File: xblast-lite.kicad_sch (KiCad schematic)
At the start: 15 parts, among them J1 TC2050, J2 XBOX LPC, J3 GPIO, J4 LCD, J5 PLCC-32 Socket, U1 74LVC125, U2 SST49LF080A-33-4C-NHE, U3 XC9572XL-xxVQx44, U4 TPS27081A

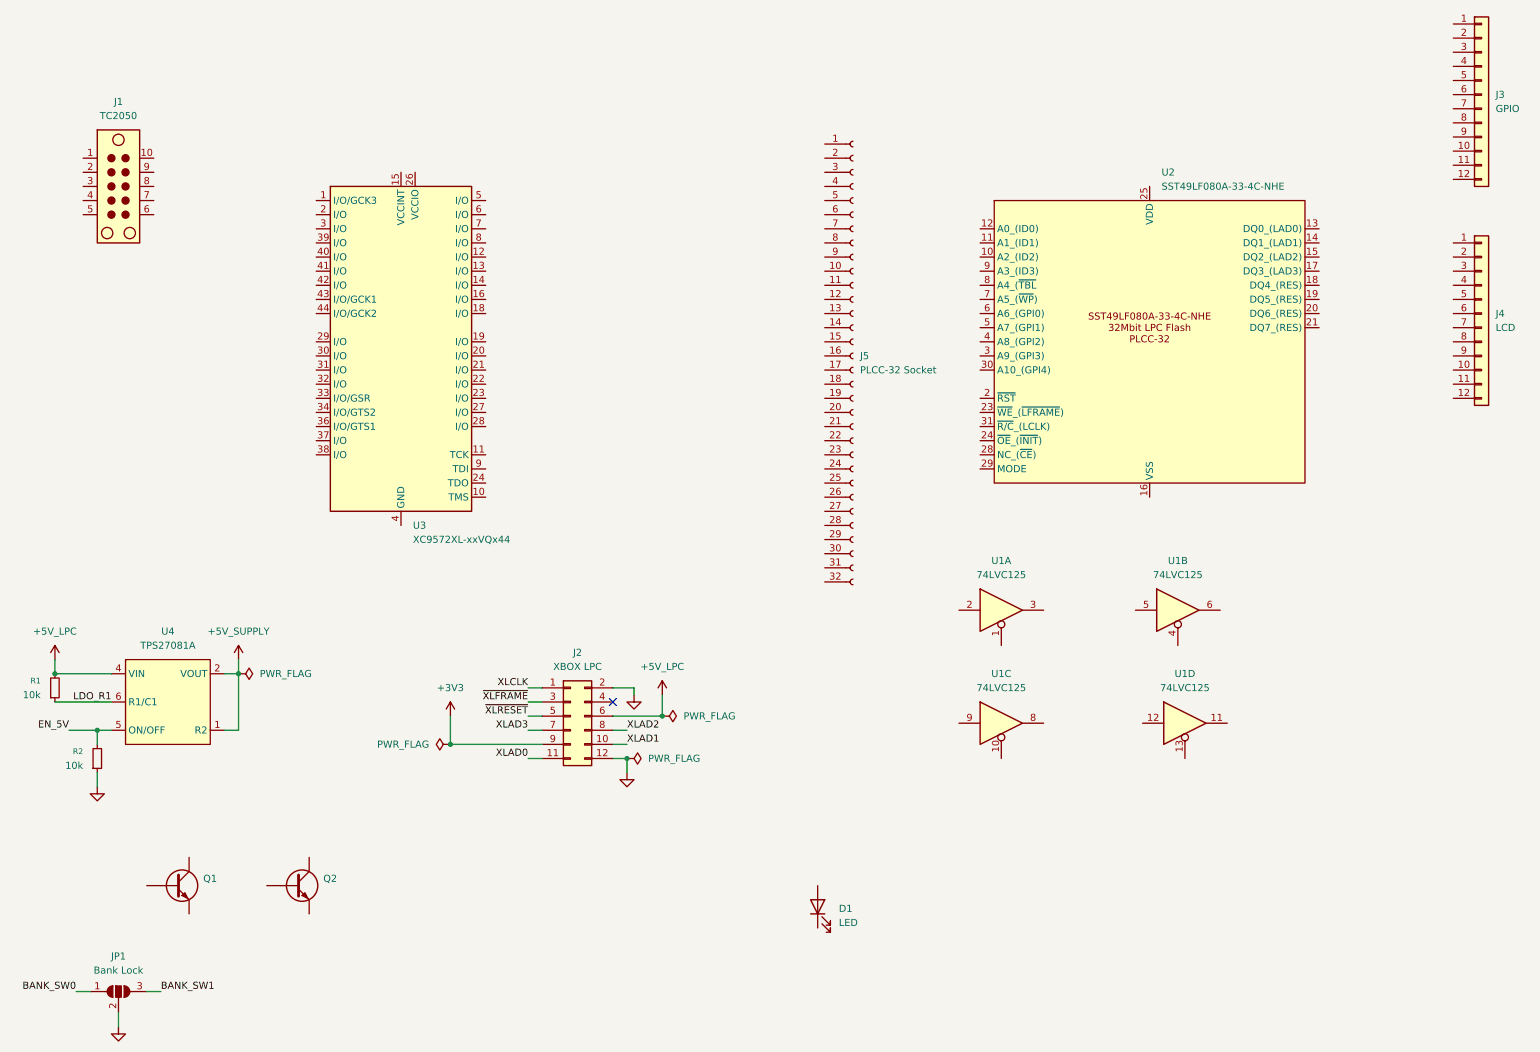
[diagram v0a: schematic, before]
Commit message: More work, initial layout
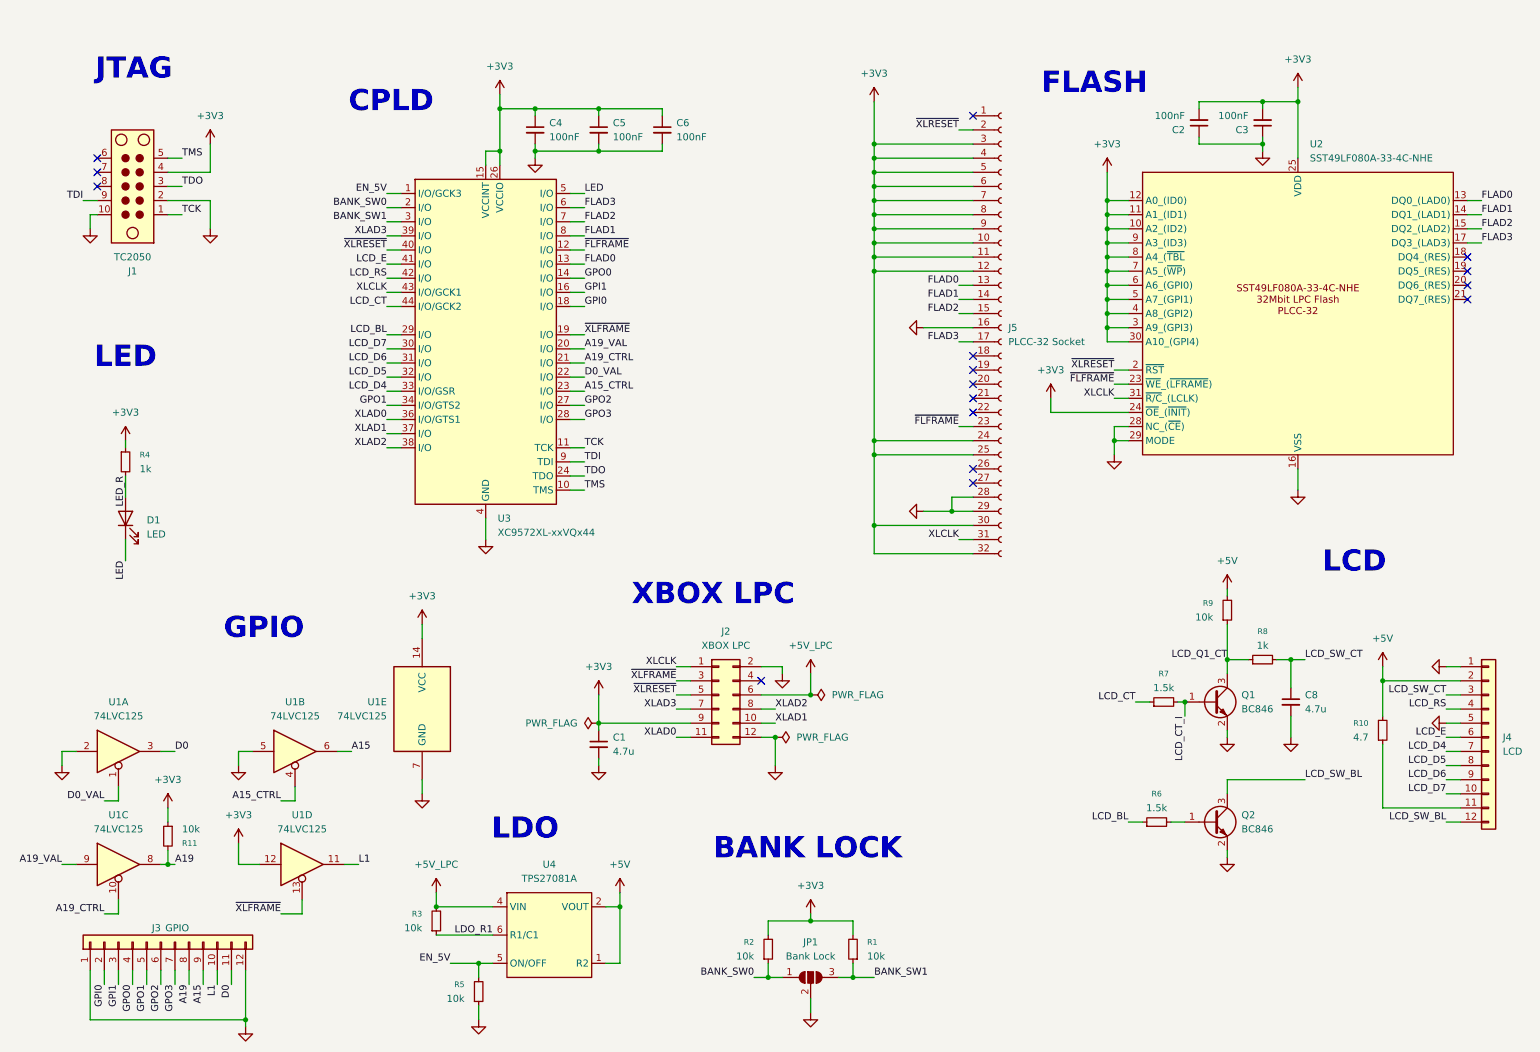
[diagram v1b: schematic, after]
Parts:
- added C1, C8: 4.7u, Capacitor_SMD:C_0805_2012Metric, symbol Device:C_Small
- added C2, C3, C4, C5, C6: 100nF, Capacitor_SMD:C_0603_1608Metric, symbol Device:C_Small
- added R1, R11, R2, R9: 10k, Resistor_SMD:R_0603_1608Metric, symbol Device:R_Small
- added R10: 4.7, Resistor_SMD:R_0805_2012Metric, symbol Device:R_Small
- added R4, R8: 1k, Resistor_SMD:R_0603_1608Metric, symbol Device:R_Small
- added R6, R7: 1.5k, Resistor_SMD:R_0603_1608Metric, symbol Device:R_Small
- added unit 5 of U1
- D1: footprint (none) -> LED_SMD:LED_0603_1608Metric; Distributor Link 1 (none) -> https://www.digikey.com/en/products/detail/liteon/LTST-C194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; Distributor Link 2 (none) -> https://www.mouser.com/en/ProductDetail/LITEON/LTST-C194KGK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; LCSC (none) -> C913102; Manufacturer (none) -> Lite-On; Manufacturer Part Number (none) -> LTST-C194KGKT
- J2: footprint Connector_PinSocket_2.54mm:PinSocket_2x06_P2.54mm_Vertical -> Connector_PinSocket_2.54mm:PinSocket_2x06_P2.54mm_Vertical_SMD; Distributor Link 1 https://www.digikey.com/en/products/detail/te-connectivity-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 -> https://www.digikey.com/en/products/detail/samtec-inc/SSM-1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; Distributor Link 2 https://www.mouser.com/en/ProductDetail/TE-Connectivity/5-5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 -> https://www.mouser.com/ProductDetail/Samtec/SSM-106-L-DV-BE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; LCSC C18078145 -> C3975151; Manufacturer Bossie -> HCTL; Manufacturer Part Number BX-PM2.54-2-6PY -> PM254-2-06-S-8.5
- J3: footprint Connector_PinSocket_2.54mm:PinSocket_1x12_P2.54mm_Vertical -> xblast-lite:SolderWirePad_1x12_SMD_2x4mm; now left out of the parts list
- Q1, Q2: value (none) -> BC846; symbol Device:Q_NPN -> Transistor_BJT:BC846
- renumbered R1 to R3, R2 to R5
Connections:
- net +5V_SUPPLY is gone; now on net +5V: U4.1 (R2), U4.2 (VOUT), U4.3 (VOUT)
- net +3V3: now also J1.4, J5.10 (Pin_10), J5.11 (Pin_11), J5.12 (Pin_12), J5.24 (Pin_24), J5.25 (Pin_25), J5.3 (Pin_3), J5.30 (Pin_30), J5.32 (Pin_32), J5.4 (Pin_4), J5.5 (Pin_5), J5.6 (Pin_6), J5.7 (Pin_7), J5.8 (Pin_8), J5.9 (Pin_9), U1.12, U2.10 (A2_(ID2)), U2.11 (A1_(ID1)), U2.12 (A0_(ID0)), U2.24 (~{OE}_(~{INIT})), U2.25 (VDD), U2.3 (A9_(GPI3)), U2.30 (A10_(GPI4)), U2.32 (VDD), U2.4 (A8_(GPI2)), U2.5 (A7_(GPI1)), U2.6 (A6_(GPI0)), U2.7 (A5_(~{WP})), U2.8 (A4_(~{TBL}), U2.9 (A3_(ID3)), U3.15 (VCCINT), U3.26 (VCCIO), U3.35 (VCCINT), C1.1, C2.2, C3.2, C4.1, C5.1, C6.1, R1.2, R11.1, R2.2, R4.1, U1.14 (VCC)
- net BANK_SW0: now also U3.2 (I/O), R2.1
- net BANK_SW1: now also U3.3 (I/O), R1.1
- net EN_5V: now also U3.1 (I/O/GCK3)
- net GND: now also J1.10, J1.2, J3.1 (Pin_1), J3.12 (Pin_12), J4.1 (Pin_1), J4.5 (Pin_5), J5.16 (Pin_16), J5.28 (Pin_28), J5.29 (Pin_29), Q1.2 (E), Q2.2 (E), U1.2, U1.5, U2.16 (VSS), U2.28 (NC_(~{CE})), U2.29 (MODE), U3.17 (GND), U3.25 (GND), U3.4 (GND), C1.2, C2.1, C3.1, C4.2, C5.2, C6.2, C8.2, U1.7 (GND)
- net XLAD0: now also U3.36 (I/O/GTS1)
- net XLAD1: now also U3.37 (I/O)
- net XLAD2: now also U3.38 (I/O)
- net XLAD3: now also U3.39 (I/O)
- net XLCLK: now also J5.31 (Pin_31), U2.31 (~{R/C}_(LCLK)), U3.43 (I/O/GCK1)
- net ~{XLFRAME}: now also U1.13, U3.19 (I/O)
- net ~{XLRESET}: now also J5.2 (Pin_2), U2.2 (~{RST}), U3.40 (I/O)
- net LED: now reaches D1.1 (K)
- net LED: now also U3.5 (I/O)
- net LED_R: now reaches D1.2 (A)
- net LED_R: now also R4.2
- net FLAD0: now reaches J5.13 (Pin_13)
- net FLAD0: now also U2.13 (DQ0_(LAD0)), U3.13 (I/O)
- net FLAD1: now reaches J5.14 (Pin_14)
- net FLAD1: now also U2.14 (DQ1_(LAD1)), U3.8 (I/O)
- net FLAD2: now reaches J5.15 (Pin_15)
- net FLAD2: now also U2.15 (DQ2_(LAD2)), U3.7 (I/O)
- net FLAD3: now reaches J5.17 (Pin_17)
- net FLAD3: now also U2.17 (DQ3_(LAD3)), U3.6 (I/O)
- net ~{FLFRAME}: now reaches J5.23 (Pin_23)
- net ~{FLFRAME}: now also U2.23 (~{WE}_(~{LFRAME})), U3.12 (I/O)
- net A15_CTRL: now reaches U1.4
- net A15_CTRL: now also U3.23 (I/O)
- net A15: now reaches U1.6
- net A15: now also J3.9 (Pin_9)
- net L1: now reaches J3.10 (Pin_10)
- net L1: now also U1.11
- net D0: now reaches J3.11 (Pin_11)
- net D0: now also U1.3
- net GPI0: now reaches J3.2 (Pin_2)
- net GPI0: now also U3.18 (I/O)
- net GPI1: now reaches J3.3 (Pin_3)
- net GPI1: now also U3.16 (I/O)
- net GPO0: now reaches J3.4 (Pin_4)
- net GPO0: now also U3.14 (I/O)
- net GPO1: now reaches J3.5 (Pin_5)
- net GPO1: now also U3.34 (I/O/GTS2)
- net GPO2: now reaches J3.6 (Pin_6)
- net GPO2: now also U3.27 (I/O)
- net GPO3: now reaches J3.7 (Pin_7)
- net GPO3: now also U3.28 (I/O)
- net A19: now reaches J3.8 (Pin_8)
- net A19: now also U1.8, R11.2
- net A19_CTRL: now reaches U1.10
- net A19_CTRL: now also U3.21 (I/O)
- net A19_VAL: now reaches U1.9
- net A19_VAL: now also U3.20 (I/O)
- net D0_VAL: now reaches U1.1
- net D0_VAL: now also U3.22 (I/O)
- net TMS: now reaches U3.10 (TMS)
- net TMS: now also J1.5
- net TCK: now reaches U3.11 (TCK)
- net TCK: now also J1.1
- net TDO: now reaches U3.24 (TDO)
- net TDO: now also J1.3
- net LCD_BL: now reaches U3.29 (I/O)
- net LCD_BL: now also R6.1
- net LCD_D7: now reaches U3.30 (I/O)
- net LCD_D7: now also J4.10 (Pin_10)
- net LCD_D6: now reaches U3.31 (I/O)
- net LCD_D6: now also J4.9 (Pin_9)
- net LCD_D5: now reaches U3.32 (I/O)
- net LCD_D5: now also J4.8 (Pin_8)
- net LCD_D4: now reaches U3.33 (I/O/GSR)
- net LCD_D4: now also J4.7 (Pin_7)
- net LCD_E: now reaches U3.41 (I/O)
- net LCD_E: now also J4.6 (Pin_6)
- net LCD_RS: now reaches U3.42 (I/O)
- net LCD_RS: now also J4.4 (Pin_4)
- net LCD_CT: now reaches U3.44 (I/O/GCK2)
- net LCD_CT: now also R7.1
- net TDI: now reaches U3.9 (TDI)
- net TDI: now also J1.9
- net at J4.11 (Pin_11): now also R10.1
- net LCD_SW_BL: now reaches J4.12 (Pin_12)
- net LCD_SW_BL: now also Q2.3 (C)
- net +5V: now reaches J4.2 (Pin_2)
- net +5V: now also R10.2, R9.2
- net LCD_SW_CT: now reaches J4.3 (Pin_3)
- net LCD_SW_CT: now also C8.1, R8.2
- new net: Q2.1 (B), R6.2
- new net LCD_CT_I: Q1.1 (B), R7.2
- new net LCD_Q1_CT: Q1.3 (C), R8.1, R9.1
- no-connect marks 1 -> 16
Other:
- note added: "BANK LOCK"
- note added: "CPLD"
- note added: "FLASH"
- note added: "GPIO"
- note added: "JTAG"
- note added: "LCD"
- note added: "LDO"
- note added: "LED"
- note added: "XBOX LPC"
- moved on the sheet: D1, J1, J2, J3, J4, J5, JP1, R3, R5, U1A, U1B, U1C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
